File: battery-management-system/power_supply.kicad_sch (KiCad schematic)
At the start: 23 parts, among them U1 L6982C33DR, U2 L6982C33DR

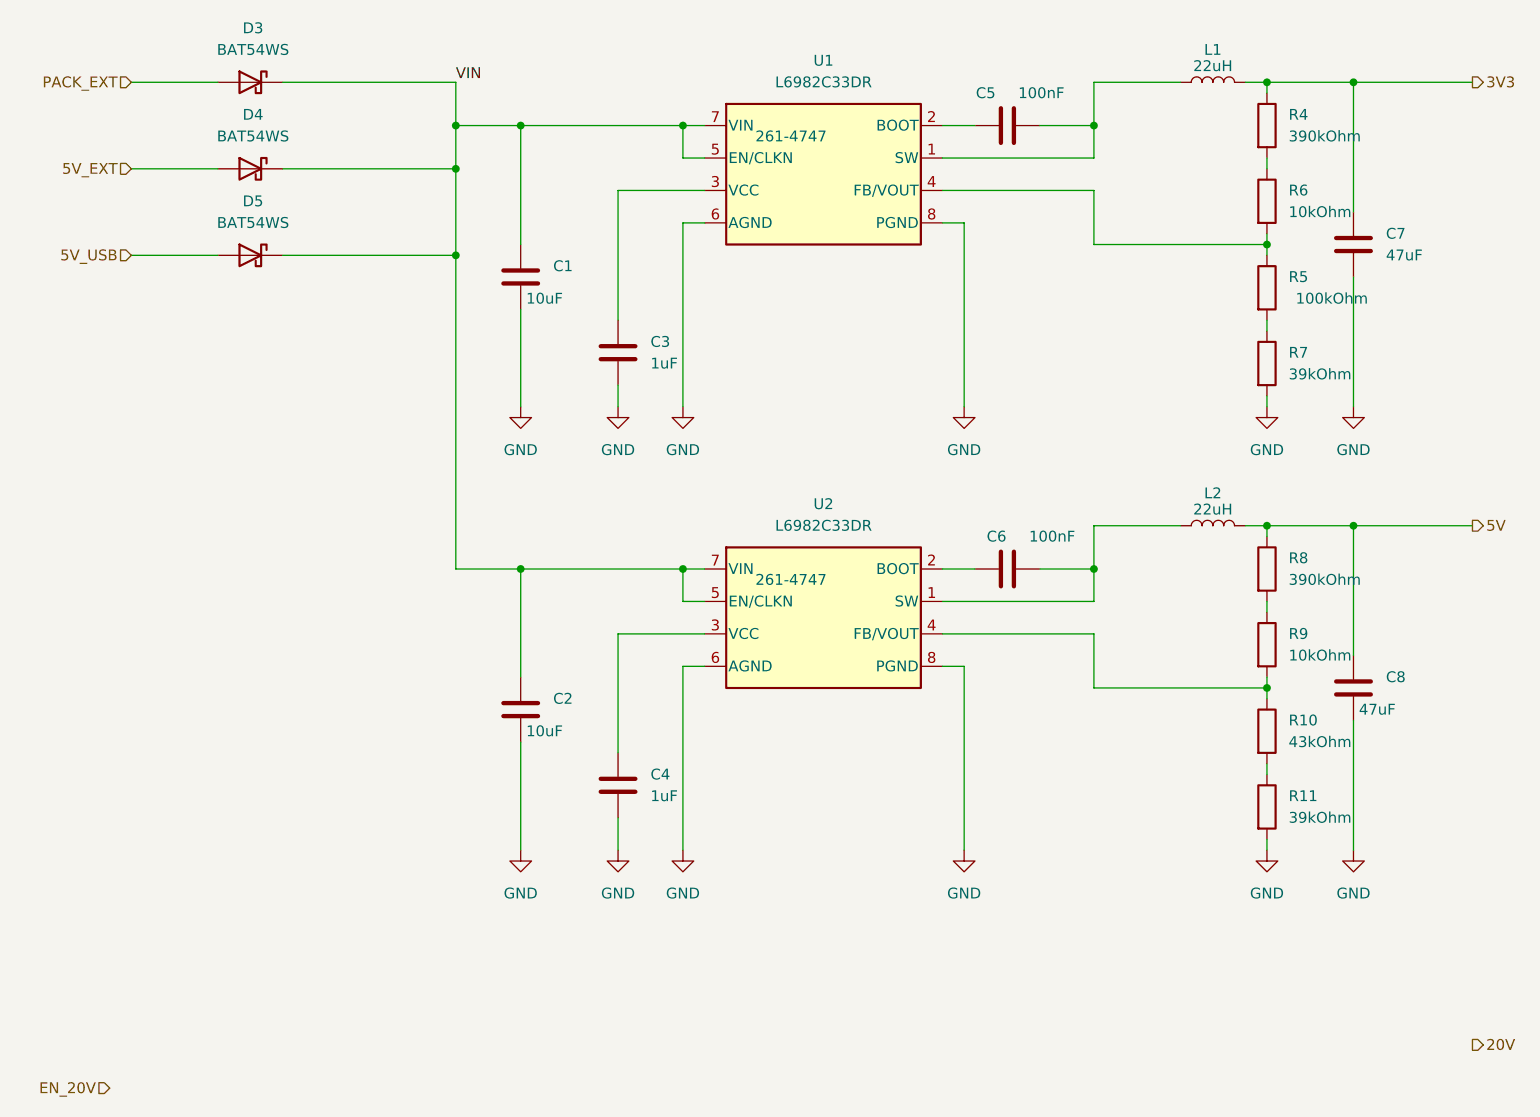
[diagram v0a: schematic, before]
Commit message: add components
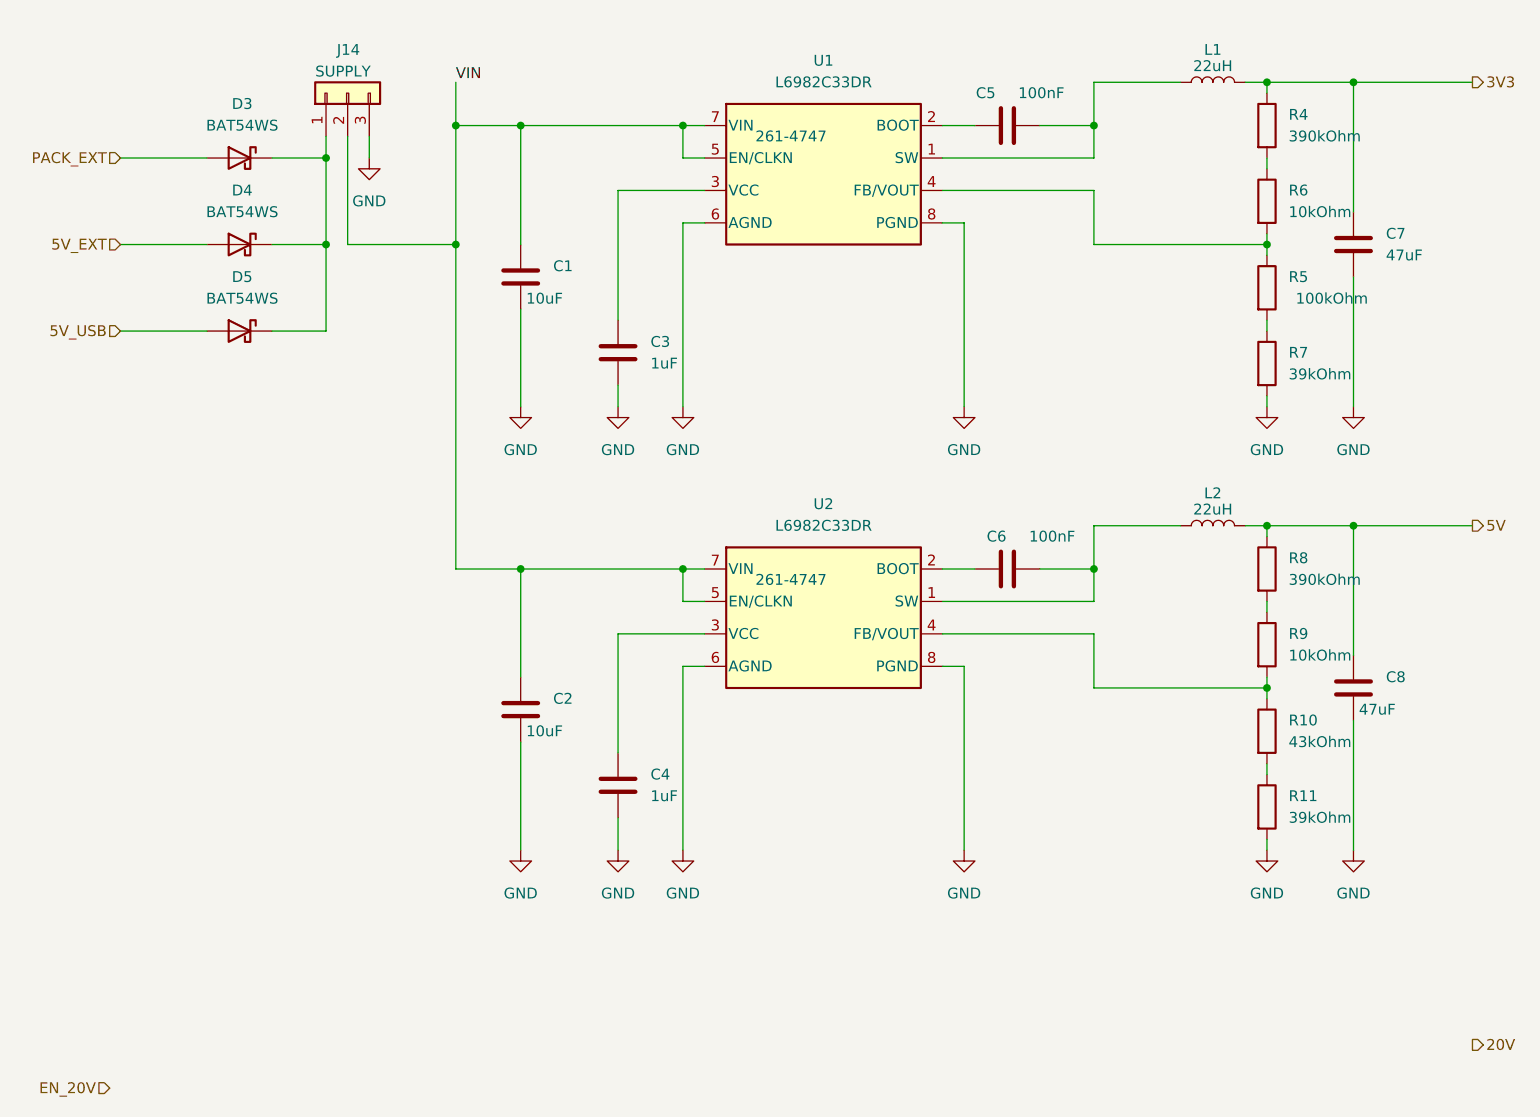
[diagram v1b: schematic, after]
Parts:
- added J14: SUPPLY, benediktibk:PinHeader_1x03_P2.54mm_Vertical, symbol benediktibk:Conn_01x03
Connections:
- net GND: now also J14.3 (Pin_3)
- net VIN: now also J14.2 (Pin_2); no longer D3.1 (K), D4.1 (K), D5.1 (K)
- new net: D3.1 (K), D4.1 (K), D5.1 (K), J14.1 (Pin_1)
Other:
- moved on the sheet: D3, D4, D5
